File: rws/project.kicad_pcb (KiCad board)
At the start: 2 copper layers, 34.6 x 30.4 mm, 10 parts, among them J1 Conn_02x09_Odd_Even, J2 Conn_02x09_Odd_Even, J3 BH1750, J4 BME280, J5 esp32-sol shield, J6 LoRa shield, J7 off/on

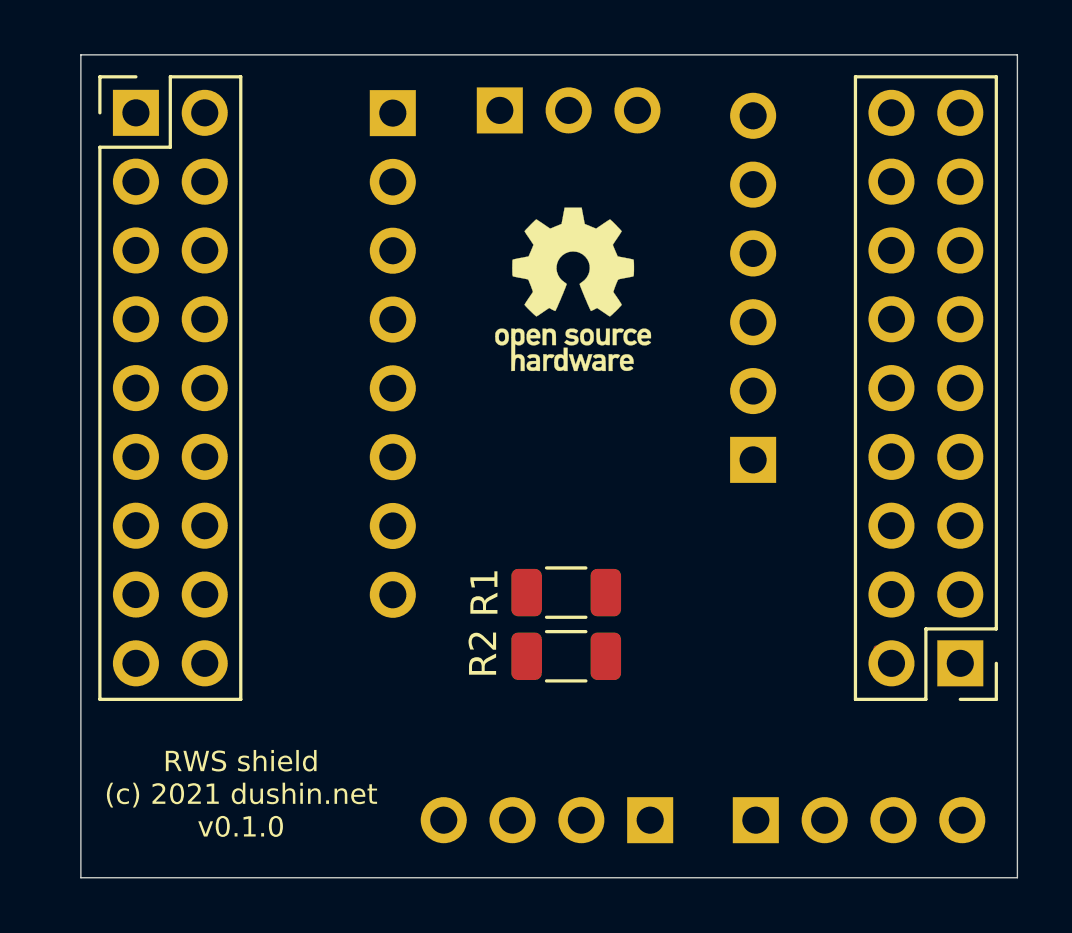
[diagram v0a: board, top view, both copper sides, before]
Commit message: Fixup and wiring of rws
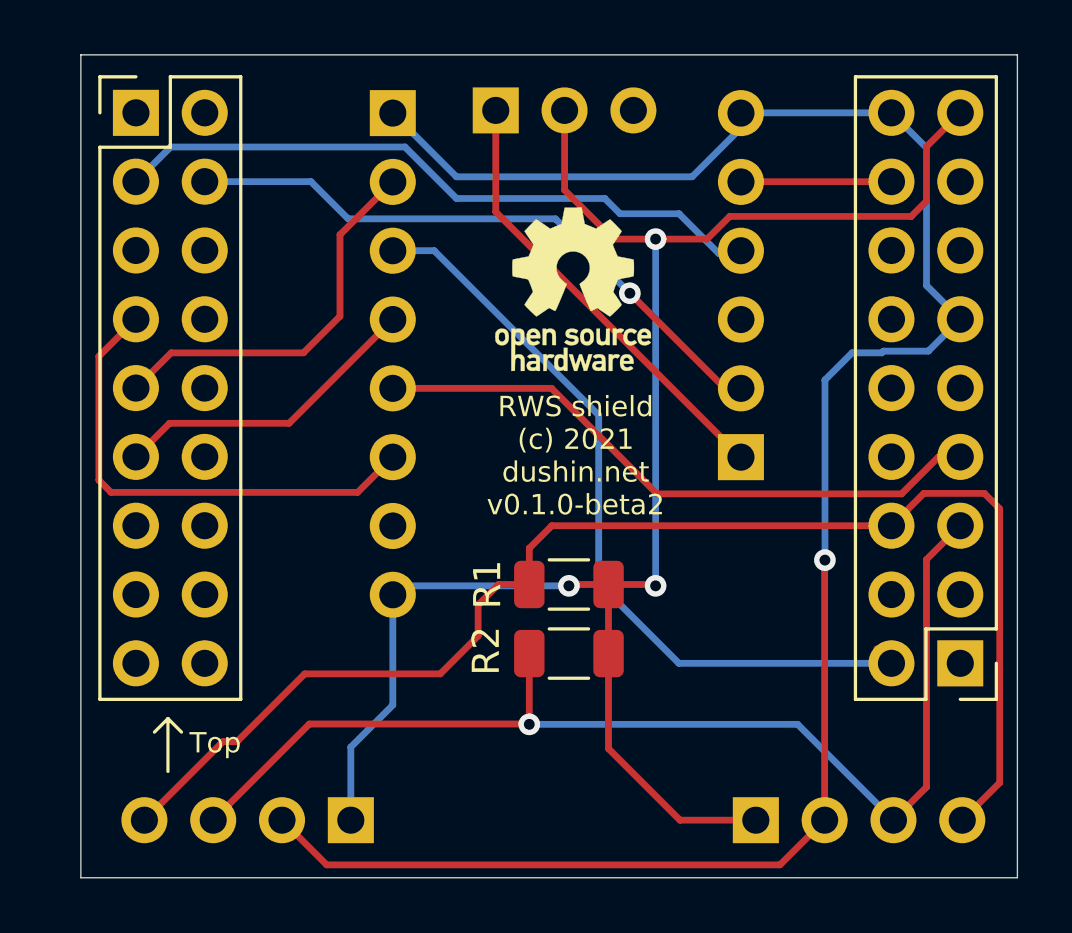
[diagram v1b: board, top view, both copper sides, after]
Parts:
- J7: value off/on -> off|on
- moved J3 11.0 mm to (135.4, 114.5)
- moved J5 0.46 mm to (149.8, 101.1)
- moved R1 0.32 mm to (143.5, 105.8)
- moved J7 0.15 mm to (140.8, 88.3)
- moved R2 0.14 mm to (143.5, 108.4)
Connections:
- J5 pad 3: /IO35 -> Net-(J5-Pad3)
- J5 pad 4: Net-(J5-Pad4) -> /IO35
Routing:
- net /GND: track 0.00 -> 72.7 mm, vias 0 -> 1
- net /VDD: track 0.00 -> 65.6 mm, vias 0 -> 3
- net /IO16: track 0.00 -> 50.3 mm
- net /IO17: track 0.00 -> 42.6 mm, vias 0 -> 1
- net /IO15: track 0.94 -> 29.3 mm
- net /IO35: track 0.00 -> 24.9 mm
- net /IO34: track 0.00 -> 23.4 mm, vias 0 -> 1
- net /IO18: track 0.00 -> 23.1 mm
- net /IO26: track 0.00 -> 18.1 mm
- net /VDD-IN: track 0.00 -> 16.9 mm
- net /IO14: track 0.00 -> 14.4 mm
- net /IO13: track 0.00 -> 11.6 mm
- net /EN: track 0.00 -> 5.72 mm
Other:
- board text added: "02|15"
- board text added: "04|00"
- board text added: "12|13"
- board text added: "14"
- board text added: "15"
- board text added: "16"
- board text added: "17"
- board text added: "17|16"
- board text added: "18"
- board text added: "18|05"
- board text added: "21|19"
- board text added: "25|26"
- board text added: "26"
- board text added: "27|14"
- board text added: "32|33"
- board text added: "34"
- board text added: "34|35"
- board text added: "35"
- board text added: "CMD|CLK"
- board text added: "EN"
- board text added: "GND"
- board text added: "GND|22"
- board text added: "NC"
- board text added: "RWS shield (c) 2021 dushin.net v0.1.0-beta2"
- board text added: "RX|23"
- board text added: "SD0|SD1"
- board text added: "SD2|SD3"
- board text added: "SVP|SVN"
- board text added: "TX|EN"
- board text added: "Top"
- board text added: "VDD"
- board text added: "VDD|GND"
- board text removed: "RWS shield (c) 2021 dushin.net v0.1.0"
